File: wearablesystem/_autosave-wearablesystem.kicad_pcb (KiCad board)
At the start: 2 copper layers, 100.5 x 99.5 mm, 64 parts, among them J1 USB_C_Receptacle_USB2.0_16P, J2 Conn_01x04_Pin, J3 Conn_Coaxial, SW1 SW_Push, SW2 SW_Push, U1 ESP32-C3, U2 SPX3819M5-L-3-3, U3 SPX3819M5-L-1-8, U4 MAX30102, U5 W25Q16JVUXIQ TR, U6 USBLC6-2SC6, U7 USBLC6-2SC6, Y1 40Mhz

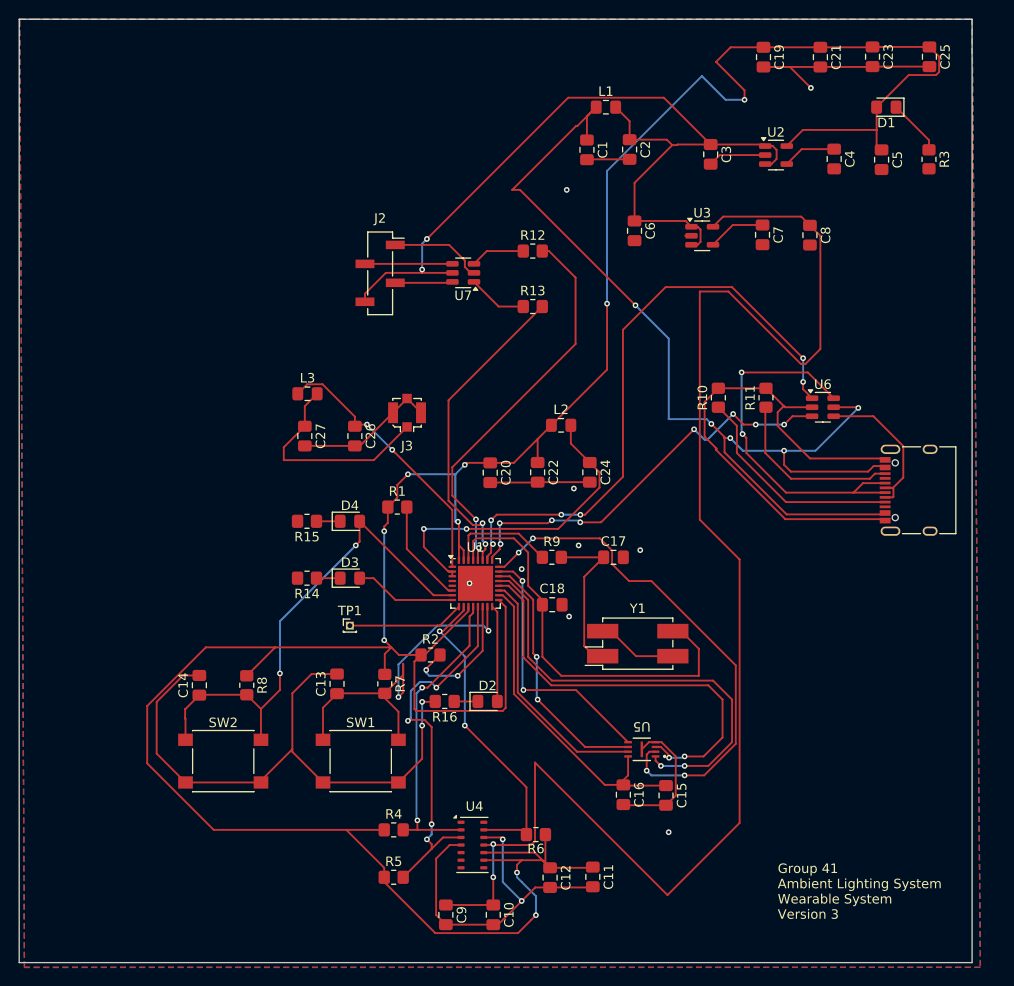
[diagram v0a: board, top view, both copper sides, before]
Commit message: updated
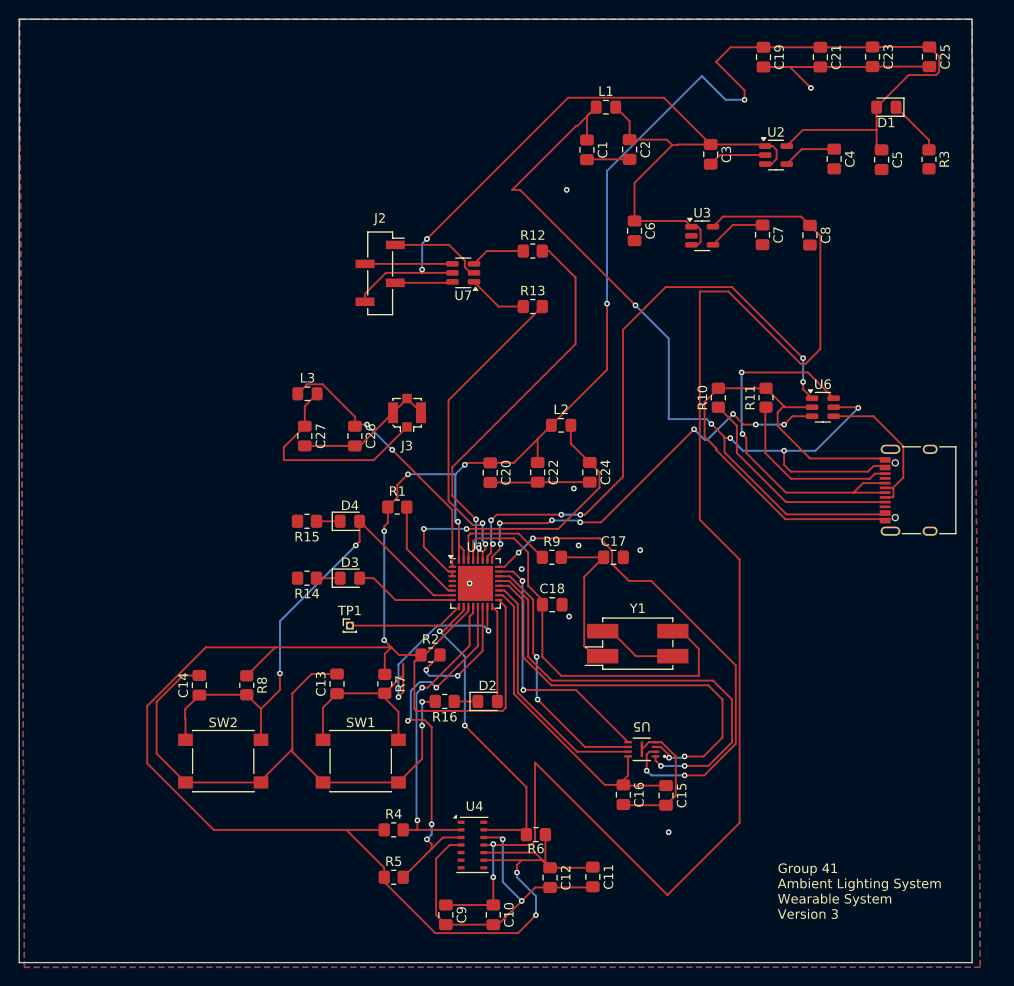
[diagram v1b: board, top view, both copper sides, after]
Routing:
- net GND: track 240.1 -> 237.2 mm
- net /XTAL_N: track 43.9 -> 42.5 mm
- net +3.3V: track 318.8 -> 317.4 mm
- net /BOOT: track 41.1 -> 40.1 mm
- net Net-(C17-Pad1): track 17.1 -> 16.2 mm
- net Net-(Y1-Pad2): track 8.49 -> 7.61 mm
- net /CHIP_EN: track 53.1 -> 52.4 mm
